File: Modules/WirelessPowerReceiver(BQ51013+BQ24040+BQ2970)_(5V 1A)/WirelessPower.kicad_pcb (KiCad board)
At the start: 4 copper layers, 56 x 56 mm, 46 parts, among them J1 Conn_01x01_Female, J2 Conn_01x01_Female, J3 Conn_01x01_Female, J4 Conn_01x01_Female, J5 BAT, J6 AC, J7 Conn_01x14, U1 BQ2971, U2 BQ51013BRHLR, U3 CSD16406Q3, U4 CSD16406Q3, U5 BQ24040DSQT

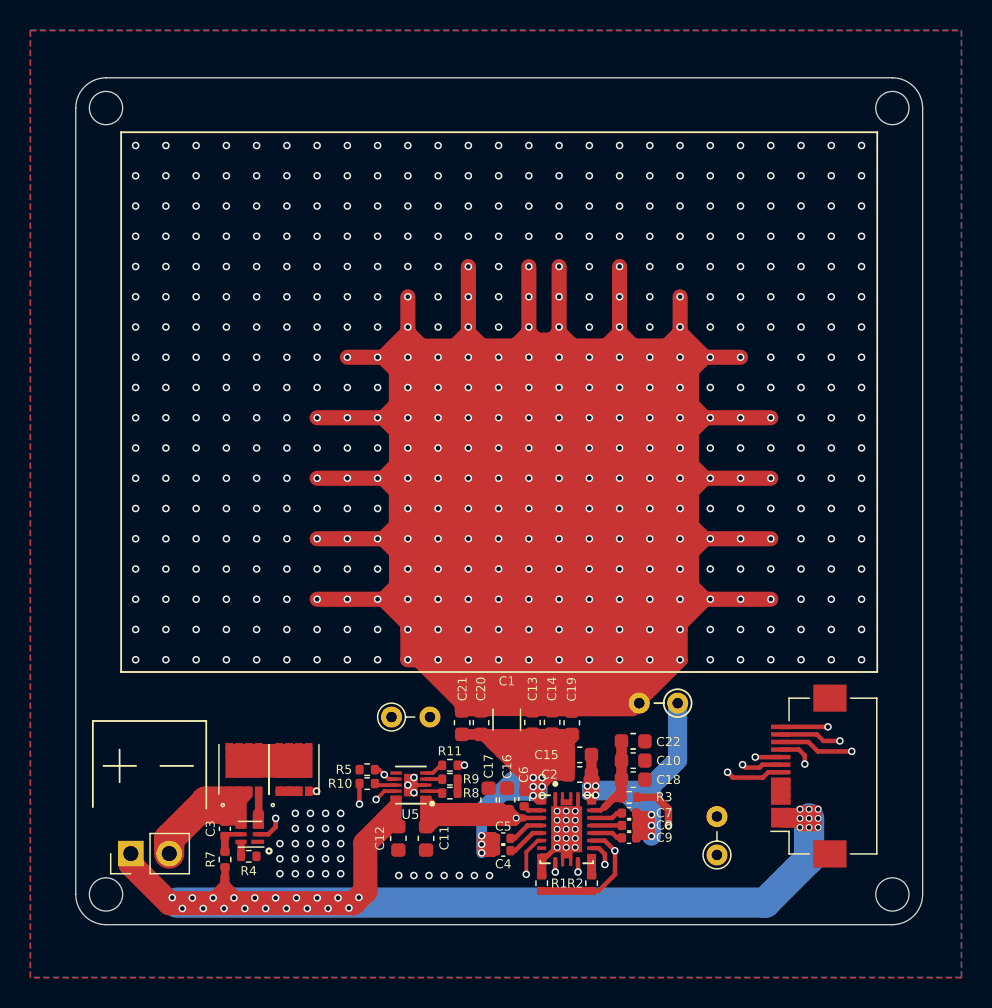
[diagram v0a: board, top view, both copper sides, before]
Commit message: Sort Out
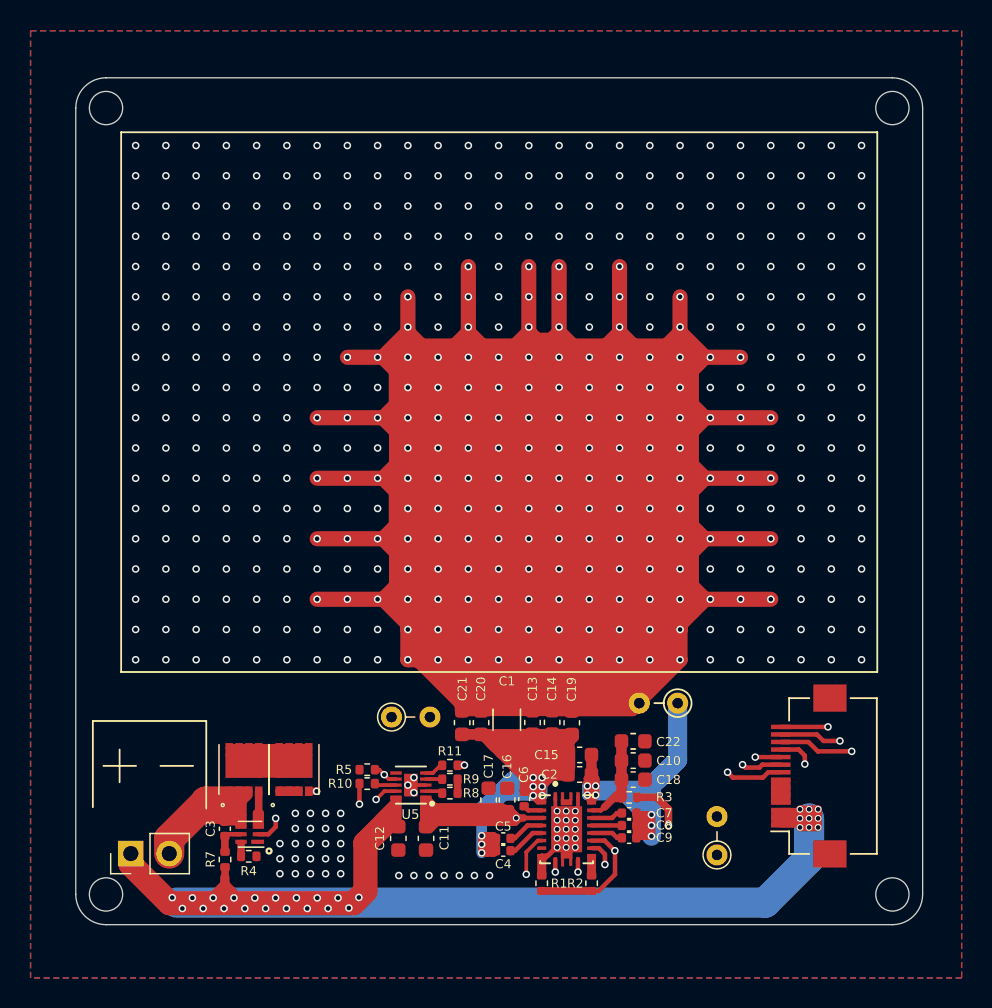
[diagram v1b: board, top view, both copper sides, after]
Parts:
- U2: footprint BQ51013B:IC_MSP430FR2522IRHLR -> lib:BQ51013BRHLR
- U3, U4: footprint BC:CSD16406Q3 -> lib:CSD16406Q3
- U5: footprint BQ24040:SON40P200X200X80-11N -> lib:BQ24040DSQT
